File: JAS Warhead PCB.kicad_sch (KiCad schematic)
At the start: 30 parts, among them CN1 DB910-7.62-2P, CN11 DB910-7.62-2P, CN12 DB910-7.62-2P, CN2 DB910-7.62-2P, CN3 DB910-7.62-2P, CN4 DB910-7.62-2P, CN5 DB910-7.62-2P, CN6 DB910-7.62-2P, J3 Conn_01x02_Pin, J5 Conn_01x03_Pin, J6 Conn_01x03_Pin, U1 LD1117S50TR_SOT223, U17 AP2127R-3.3, U2 AHT20-F

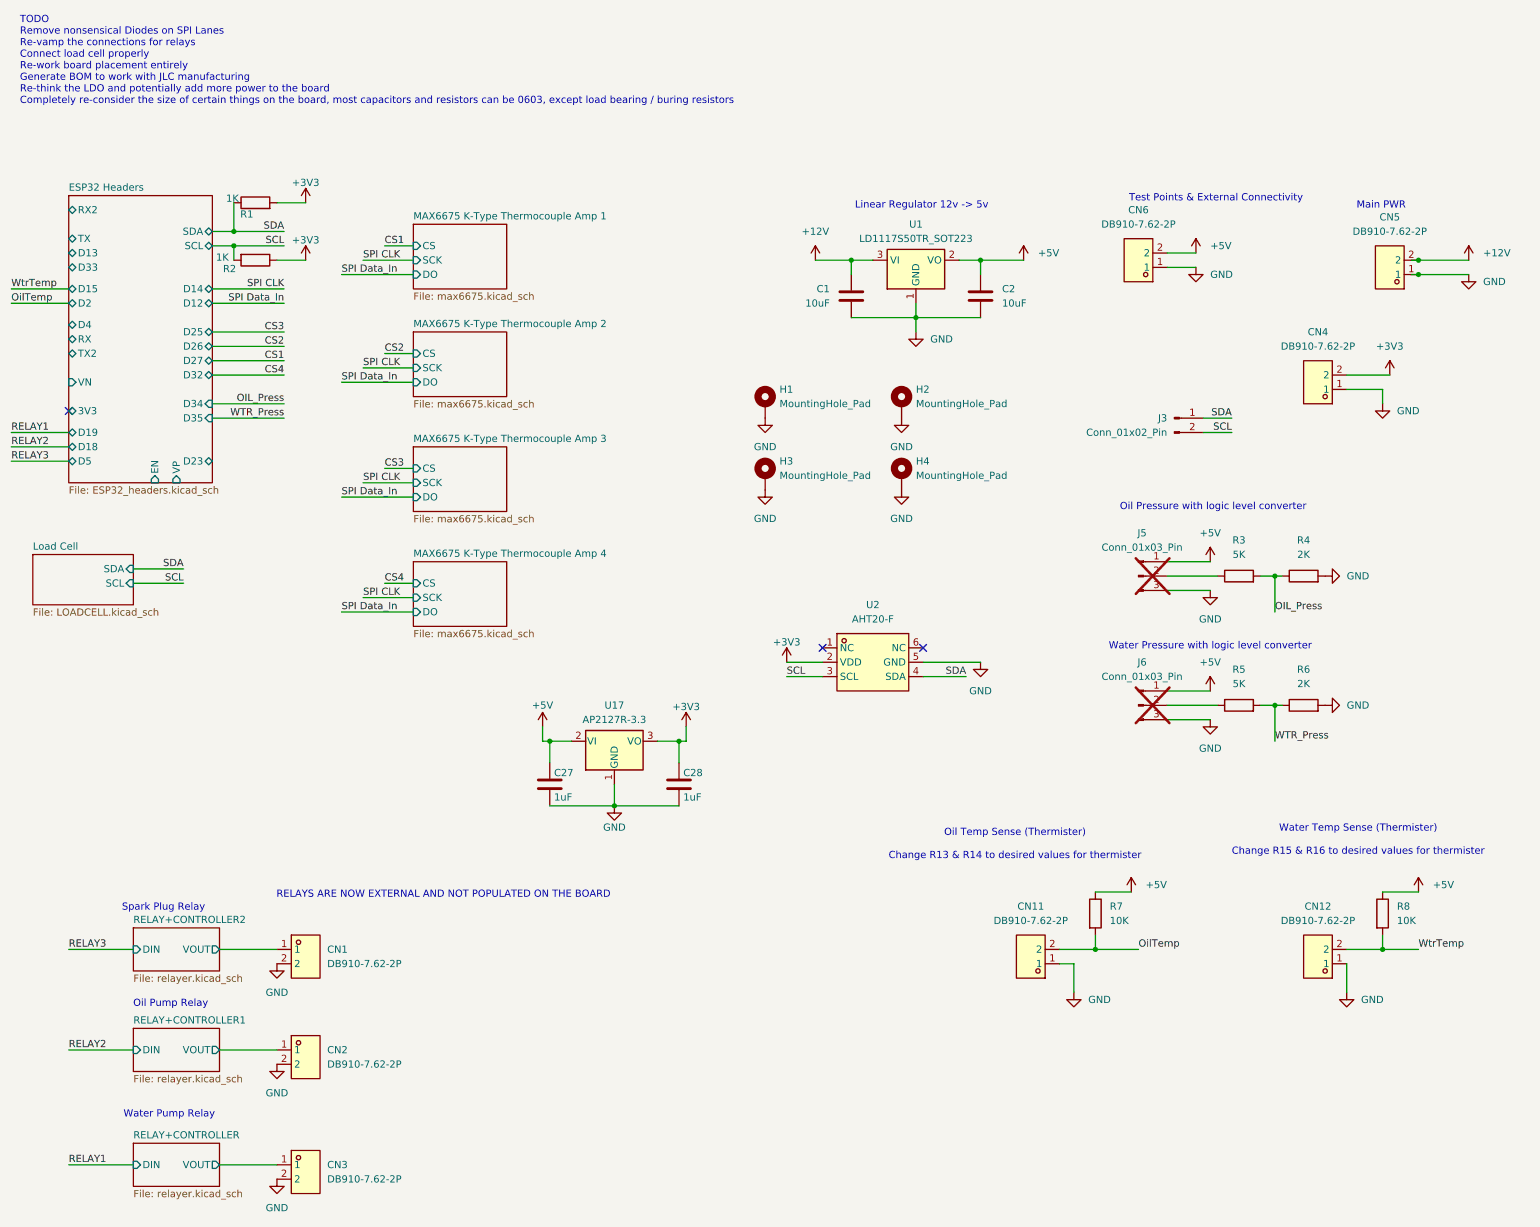
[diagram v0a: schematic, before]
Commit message: almost ready for prod
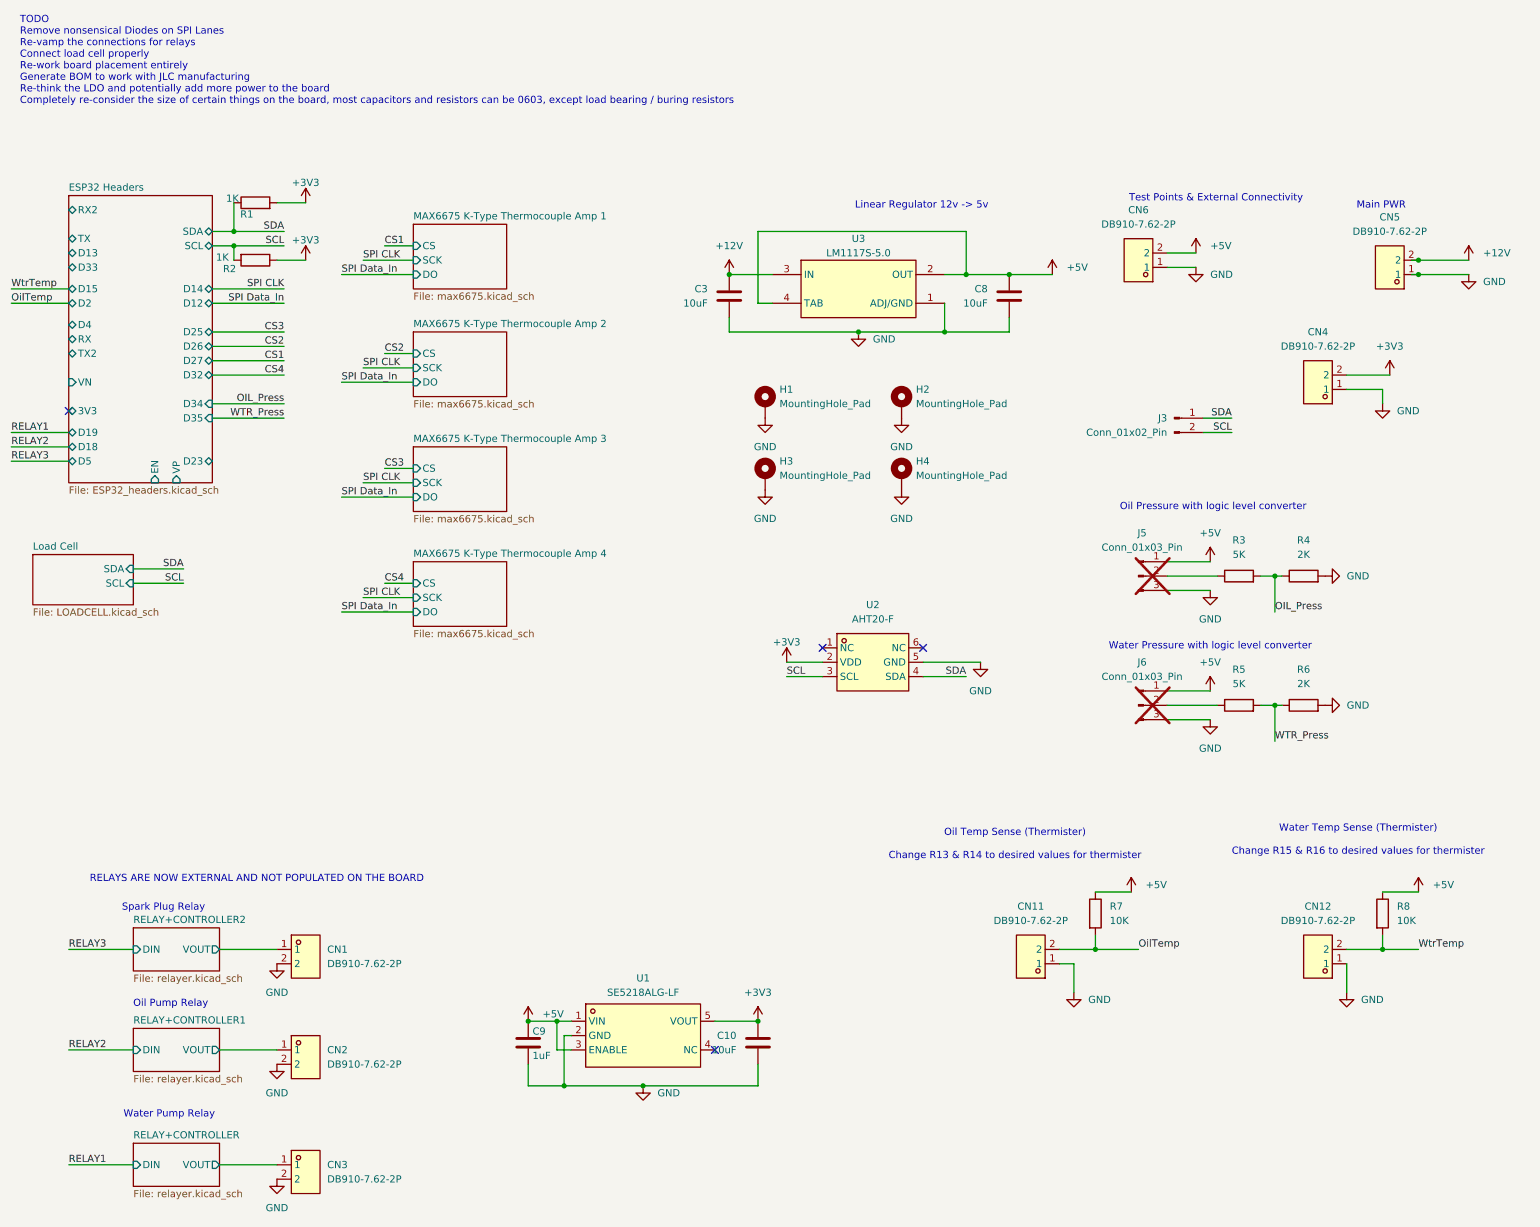
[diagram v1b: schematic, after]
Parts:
- removed C1, C2: 10uF, Capacitor_SMD:C_0402_1005Metric, symbol Device:C
- removed C27, C28: 1uF, Capacitor_SMD:C_0402_1005Metric, symbol Device:C
- removed U1: LD1117S50TR_SOT223, Package_TO_SOT_SMD:SOT-223-3_TabPin2, symbol Regulator_Linear:LD1117S50TR_SOT223
- removed U17: AP2127R-3.3, Package_TO_SOT_SMD:SOT-89-3, symbol Regulator_Linear:AP2127R-3.3
- added C10, C3, C8: 10uF, Capacitor_SMD:C_0603_1608Metric, symbol Device:C
- added C9: 1uF, Capacitor_SMD:C_0402_1005Metric, symbol Device:C
- added U1: SE5218ALG-LF, blastLib:SOT-23-5_L3.0-W1.7-P0.95-LS2.8-BR, symbol blastLib:SE5218ALG-LF
- added U3: LM1117S-5.0, blastLib:SOT-223-3_L6.5-W3.4-P2.30-LS7.0-BR, symbol blastLib:LM1117S-5.0
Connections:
- net +12V: now also C3.1, U3.3 (IN)
- net +3V3: now also C10.1, U1.5 (VOUT)
- net +5V: now also C8.1, C9.1, U1.1 (VIN), U1.3 (ENABLE), U3.2 (OUT), U3.4 (TAB)
- net GND: now also C10.2, C3.2, C8.2, C9.2, U1.2 (GND), U3.1 (ADJ/GND)
- no-connect marks 3 -> 4
